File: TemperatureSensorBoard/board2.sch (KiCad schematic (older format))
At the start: 25 parts, among them K1 CONN_3, P1 CONN_1, P2 CONN_2, P3 CONN_2, U1 LM324, U2 CD4052

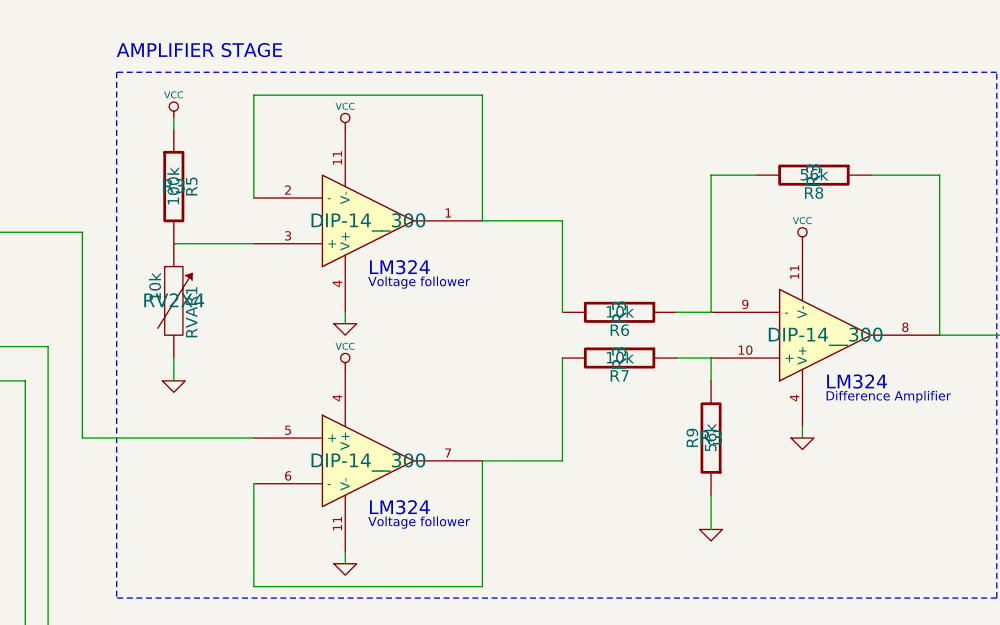
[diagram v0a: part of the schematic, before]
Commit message: Kicad
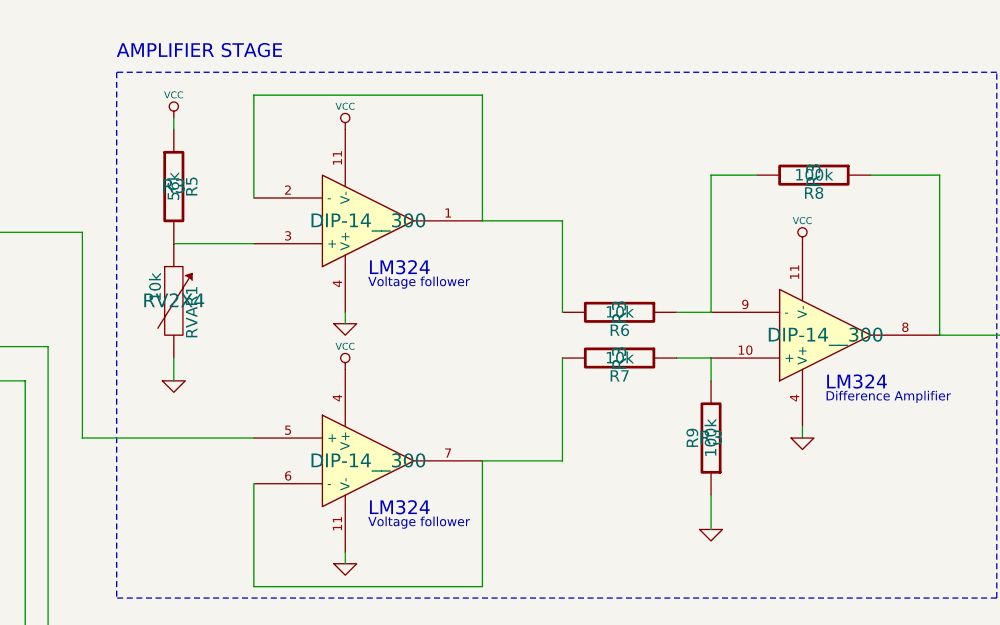
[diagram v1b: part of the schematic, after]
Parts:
- R5: value 100k -> 56k
- R8, R9: value 56k -> 100k
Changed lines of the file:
@@
 Sheet 1 1
 Title ""
-Date "3 oct 2014"
+Date "12 oct 2014"
 Rev ""
 Comp ""
@@
 P 8000 5200
 F 0 "R9" V 8080 5200 50  0000 C CNN
-F 1 "56k" V 8000 5200 50  0000 C CNN
+F 1 "100k" V 8000 5200 50  0000 C CNN
 F 2 "R3" H 8000 5200 60  0000 C CNN
 F 3 "" H 8000 5200 60  0001 C CNN
@@
 P 8450 4050
 F 0 "R8" V 8530 4050 50  0000 C CNN
-F 1 "56k" V 8450 4050 50  0000 C CNN
+F 1 "100k" V 8450 4050 50  0000 C CNN
 F 2 "R3" H 8450 4050 60  0000 C CNN
 F 3 "" H 8450 4050 60  0001 C CNN
@@
 P 5650 4100
 F 0 "R5" V 5730 4100 50  0000 C CNN
-F 1 "100k" V 5650 4100 50  0000 C CNN
+F 1 "56k" V 5650 4100 50  0000 C CNN
 F 2 "R3" H 5650 4100 60  0000 C CNN
 F 3 "" H 5650 4100 60  0001 C CNN
